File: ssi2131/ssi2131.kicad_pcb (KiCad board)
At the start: 2 copper layers, 50.4 x 108 mm, 34 parts, among them J1 Saw Out, J2 Pulse Out, J3 Tri Out, J4 Hard Sync, J5 Soft Sync, J7 16-Pin uZeus Power Header, J9 Expo Freq, U1 SSI2131, U2 LM4040DBZ-2.5

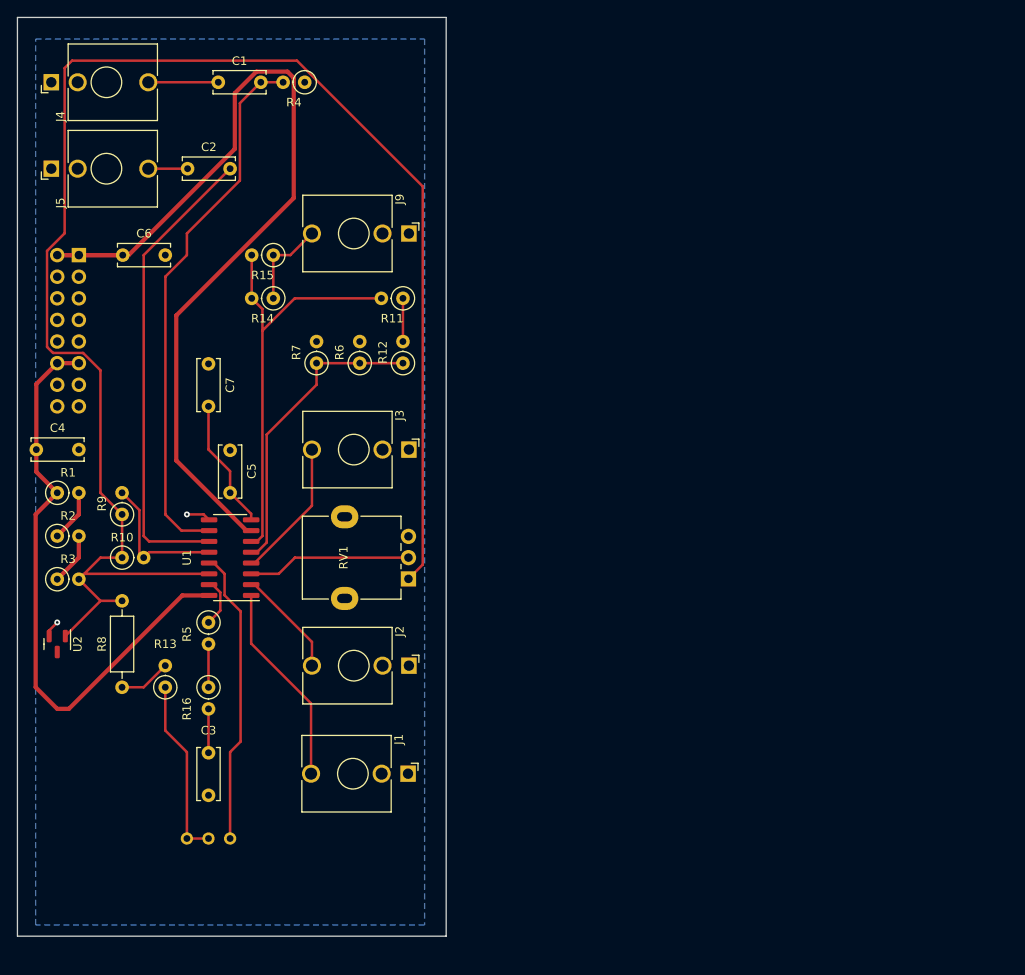
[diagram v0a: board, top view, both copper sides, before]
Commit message: rework PCB layout
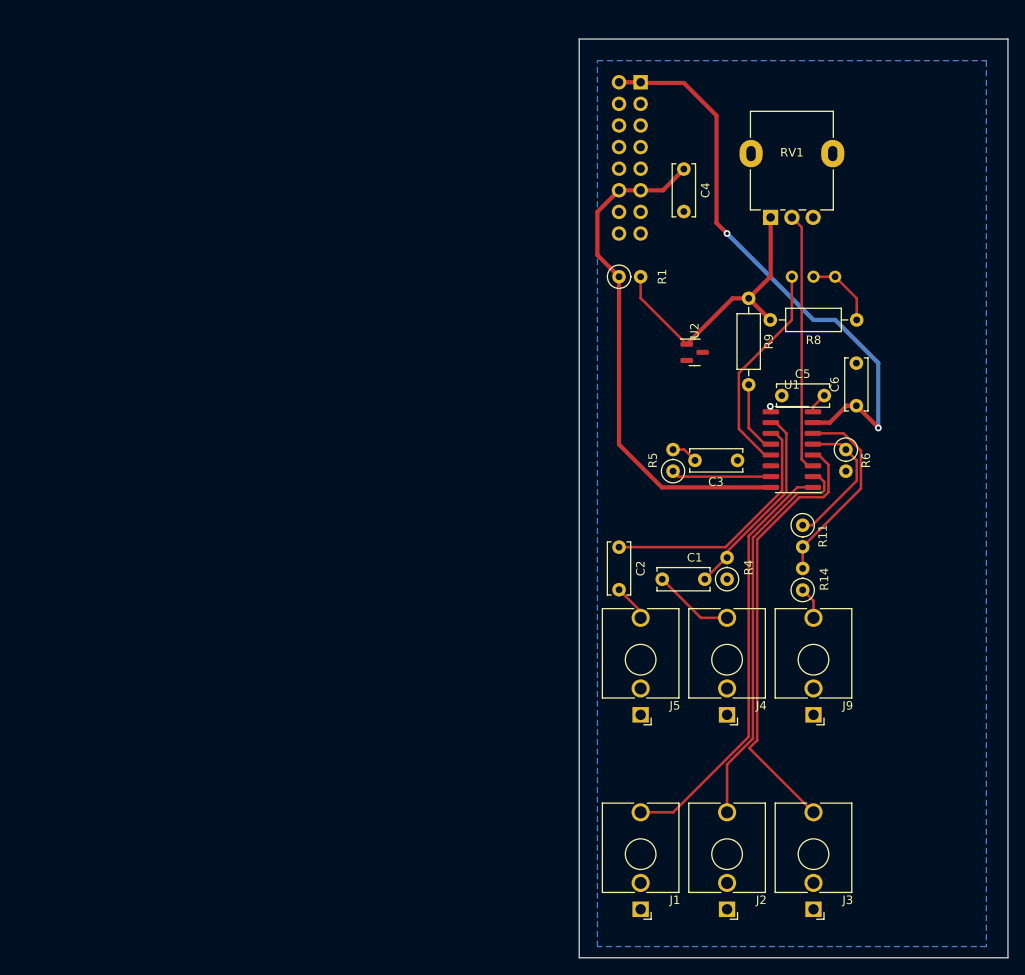
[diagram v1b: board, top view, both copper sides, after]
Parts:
- removed C7: 680 pF, Capacitor_THT:C_Disc_D6.0mm_W2.5mm_P5.00mm
- removed R10: 1 MOhms, Resistor_THT:R_Axial_DIN0207_L6.3mm_D2.5mm_P2.54mm_Vertical
- removed R12, R7: 47 kOhms, Resistor_THT:R_Axial_DIN0207_L6.3mm_D2.5mm_P2.54mm_Vertical
- removed R13: 100 Ohms, Resistor_THT:R_Axial_DIN0207_L6.3mm_D2.5mm_P2.54mm_Vertical
- removed R15: 100 kOhms, Resistor_THT:R_Axial_DIN0207_L6.3mm_D2.5mm_P2.54mm_Vertical
- removed R16: 47 Ohms, Resistor_THT:R_Axial_DIN0207_L6.3mm_D2.5mm_P2.54mm_Vertical
- removed R2: 2.2 kOhms, Resistor_THT:R_Axial_DIN0207_L6.3mm_D2.5mm_P2.54mm_Vertical
- removed R3: 1 kOhms, Resistor_THT:R_Axial_DIN0207_L6.3mm_D2.5mm_P2.54mm_Vertical
- C5: value 3.3 nF -> 3.9 nF
- R1: value 4.7 kOhms -> 7.5 kOhms
- R11: value 220 kOhms -> 267 kOhms
- R14: value 100 kOhms -> 49.9 kOhms
- R5: value 220 Ohms -> 267 Ohms
- R6: value 4.7 kOhms -> 4.3 kOhms
- R8: value 22 kOhms -> 22.1 kOhms
- R9: value 1 MOhms -> 499 kOhms; footprint Resistor_THT:R_Axial_DIN0207_L6.3mm_D2.5mm_P2.54mm_Vertical -> Resistor_THT:R_Axial_DIN0207_L6.3mm_D2.5mm_P10.16mm_Horizontal
- moved J4 108.8 mm to (172.7, 112.5), turned to 180 degrees
- moved R8 96.6 mm to (188.0, 66.0), turned to 180 degrees
- moved J5 94.5 mm to (162.6, 112.5), turned to 180 degrees
- moved RV2 93.4 mm to (180.3, 61.0), turned to 180 degrees
- moved U2 82.4 mm to (168.9, 69.8), turned to 0 degrees
- moved C6 82.2 mm to (187.9, 71.1), turned to -90 degrees
- moved C1 78.3 mm to (165.1, 96.5)
- moved R9 77.9 mm to (175.3, 63.5), turned to -90 degrees
- moved R4 76.7 mm to (172.7, 96.5), turned to 90 degrees
- moved C4 76.4 mm to (167.6, 53.3), turned to 90 degrees
- moved J9 73.9 mm to (182.9, 112.5), turned to 180 degrees
- moved C3 73.6 mm to (173.9, 82.5), turned to 180 degrees
- moved J3 72.0 mm to (182.9, 135.3), turned to 180 degrees
- moved R14 71.1 mm to (181.6, 97.8), turned to 90 degrees
- moved C5 70.8 mm to (184.2, 74.9), turned to 180 degrees
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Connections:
- C3 pad 2: Net-(C3-Pad2) -> Net-(R5-Pad2)
- R1 pad 2: Net-(R1-Pad2) -> VREF
- R11 pad 1: Net-(R11-Pad1) -> HFTrack
- R5 pad 2: Net-(R16-Pad1) -> Net-(R5-Pad2)
- R8 pad 1: Net-(R13-Pad2) -> Net-(R8-Pad1)
- RV2 pad 2: Net-(R13-Pad1) -> Net-(R8-Pad1)
- RV2 pad 3: Net-(R13-Pad1) -> Net-(R8-Pad1)
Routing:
- net VREF: track 193.2 -> 35.3 mm
- net -12V: track 111.5 -> 68.8 mm, vias 0 -> 2
- net HardSync: track 64.0 -> 23.5 mm
- net TriOut: track 16.5 -> 51.8 mm
- net PulseOut: track 12.7 -> 46.8 mm
- net ExpoFreq: track 50.7 -> 23.2 mm
- net SawOut: track 23.9 -> 49.9 mm
- net SoftSync: track 55.3 -> 29.5 mm
- net Net-(R13-Pad1): track 21.4 -> 0.00 mm
- net HFTrack: track 36.0 -> 16.8 mm
- net TCAP: track 15.4 -> 2.46 mm
- net PWMCtrl: track 19.3 -> 30.6 mm
- net +5V: track 70.7 -> 60.6 mm
- net ExpoScale: track 34.8 -> 25.5 mm
- net Net-(R8-Pad1): track 0.00 -> 8.67 mm
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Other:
- board text added: "SSI2131 Typical Application Circuit Revision 2 9/30/2022"
- board text removed: "SSI2131 Typical Application Circuit Revision 1 9/30/2022"
